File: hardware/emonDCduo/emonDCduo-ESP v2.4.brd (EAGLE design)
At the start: 114.2 x 76.5 mm, 108 parts, among them P1 B4B-PH-K, X3 GMSTBV2, X4 GMSTBV2, Y1 32Khz

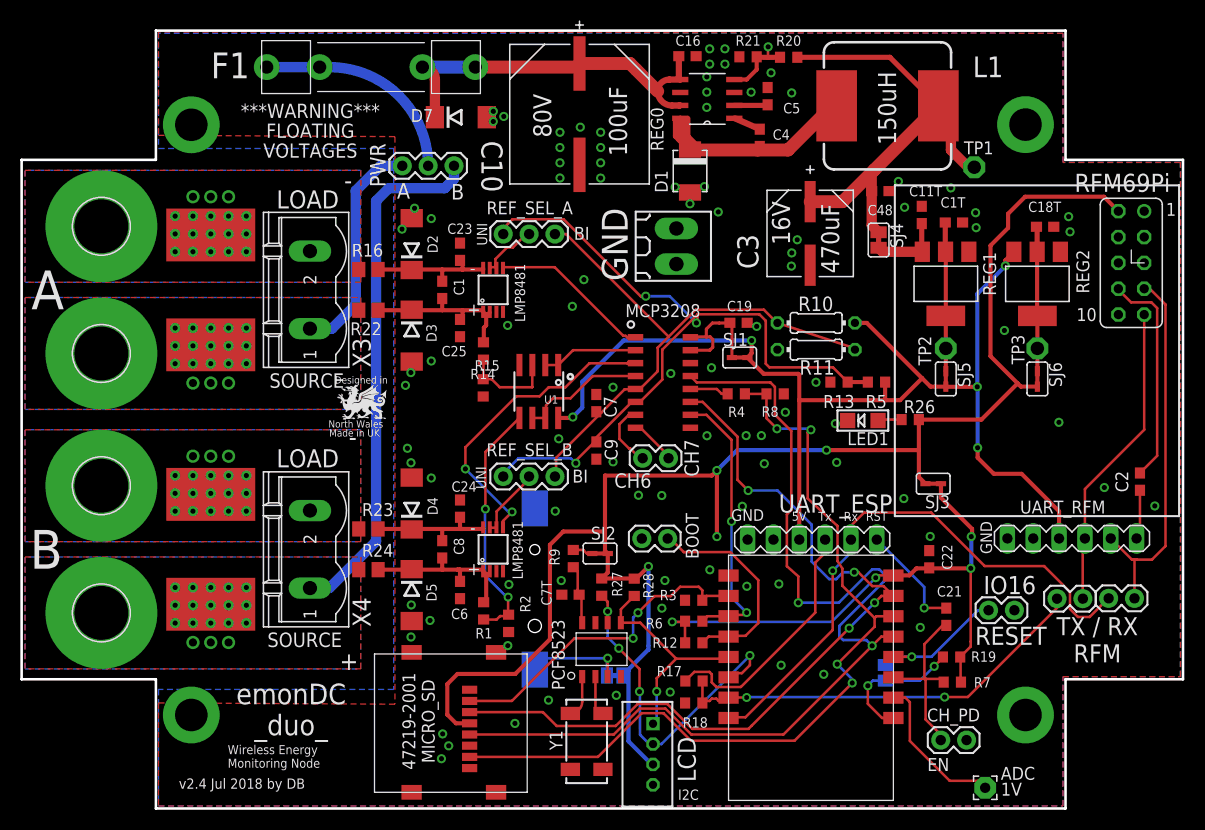
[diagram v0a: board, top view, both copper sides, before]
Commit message: commit v3.0
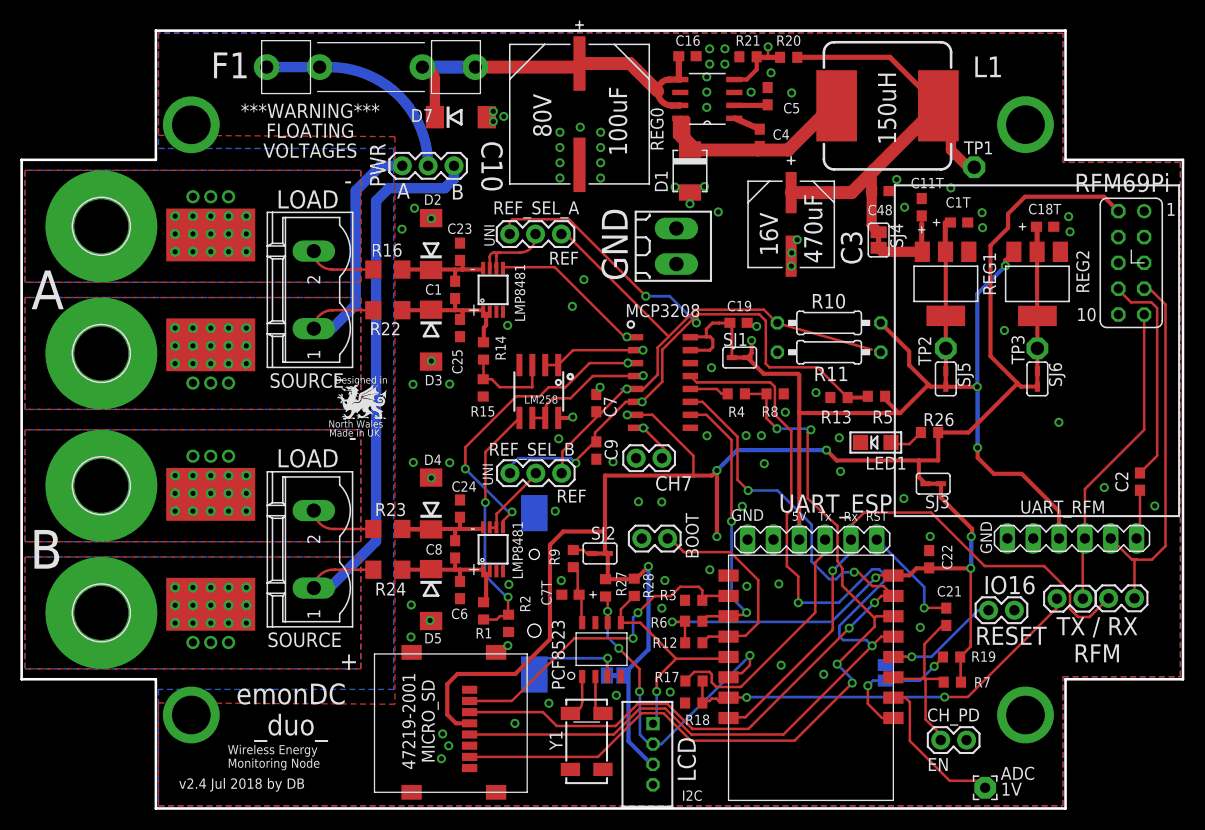
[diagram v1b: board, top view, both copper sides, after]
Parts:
- C11T, C18T, C1T: device rcl:C0603 -> rcl7:C0603POL
- C7T: device rcl@1:C0603 -> rcl7:C0603POL
- R10, R11: device rcl:0204/7 -> rcl7:0207/10
- R16, R22, R23, R24: device rcl:R0805 -> rcl7:R1206
- moved LED1 2.50 mm to (77.6, 37.7)
- moved R26 2.29 mm to (82.9, 38.7)
- moved C3 2.07 mm to (69.3, 59.2)
- moved D2 1.91 mm to (33.9, 57.2)
- moved D3 1.91 mm to (33.9, 48.2)
- moved D4 1.91 mm to (33.9, 31.8)
- moved D5 1.91 mm to (33.9, 22.8)
- moved R16 1.91 mm to (29.7, 54.8)
- moved R22 1.91 mm to (29.7, 50.8)
- moved R23 1.91 mm to (29.7, 29.2)
- moved R24 1.91 mm to (29.7, 25.2)
- moved R13 1.52 mm to (74.0, 42.2)
- moved R5 1.40 mm to (77.7, 42.3)
- moved R11 1.30 mm to (73.0, 46.6)
- moved R10 1.27 mm to (73.0, 49.5)
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- renumbered U1 to LM258
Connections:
- removed net CH6: J5.2, MCP3208.7
- net +3V3: now also MCP3208.7
- net GND: now also J5.2
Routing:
- net +5V: track 111.5 -> 88.9 mm
- net +3V3: track 159.3 -> 168.7 mm, vias 4 -> 5
- net LOAD-NEG-A: track 0.00 -> 6.60 mm
- net LOAD-NEG-B: track 0.00 -> 6.53 mm
- net CH6: track 6.47 -> 0.00 mm
- net SOURCE-POS-A: track 22.3 -> 28.5 mm
- net SOURCE-POS-B: track 51.7 -> 57.9 mm
- net REF_A_INPUT: track 5.91 -> 8.98 mm
- net SOURCE-POS-B_T: track 17.0 -> 14.4 mm
- net SOURCE-POS-A_T: track 16.6 -> 14.2 mm
- net LOAD-NEG-A_T: track 12.8 -> 10.5 mm
- net CH7: track 4.65 -> 6.37 mm, vias 0 -> 1
- net PRE_6.5V: track 46.7 -> 48.2 mm
- net SCL: track 35.9 -> 34.5 mm
- net BI_REF: track 55.7 -> 56.9 mm, vias 0 -> 1
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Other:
- board text added: "REF"
- board text removed: "BI"
- board text removed: "CH6"
